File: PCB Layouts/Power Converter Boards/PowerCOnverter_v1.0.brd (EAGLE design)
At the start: 100 x 80 mm, 47 parts, among them Q1 PMBT3906, Q2 PMBT3906, Q3 PMBT3906, X1 48V, X2 12V, X3 24V, X4 15V

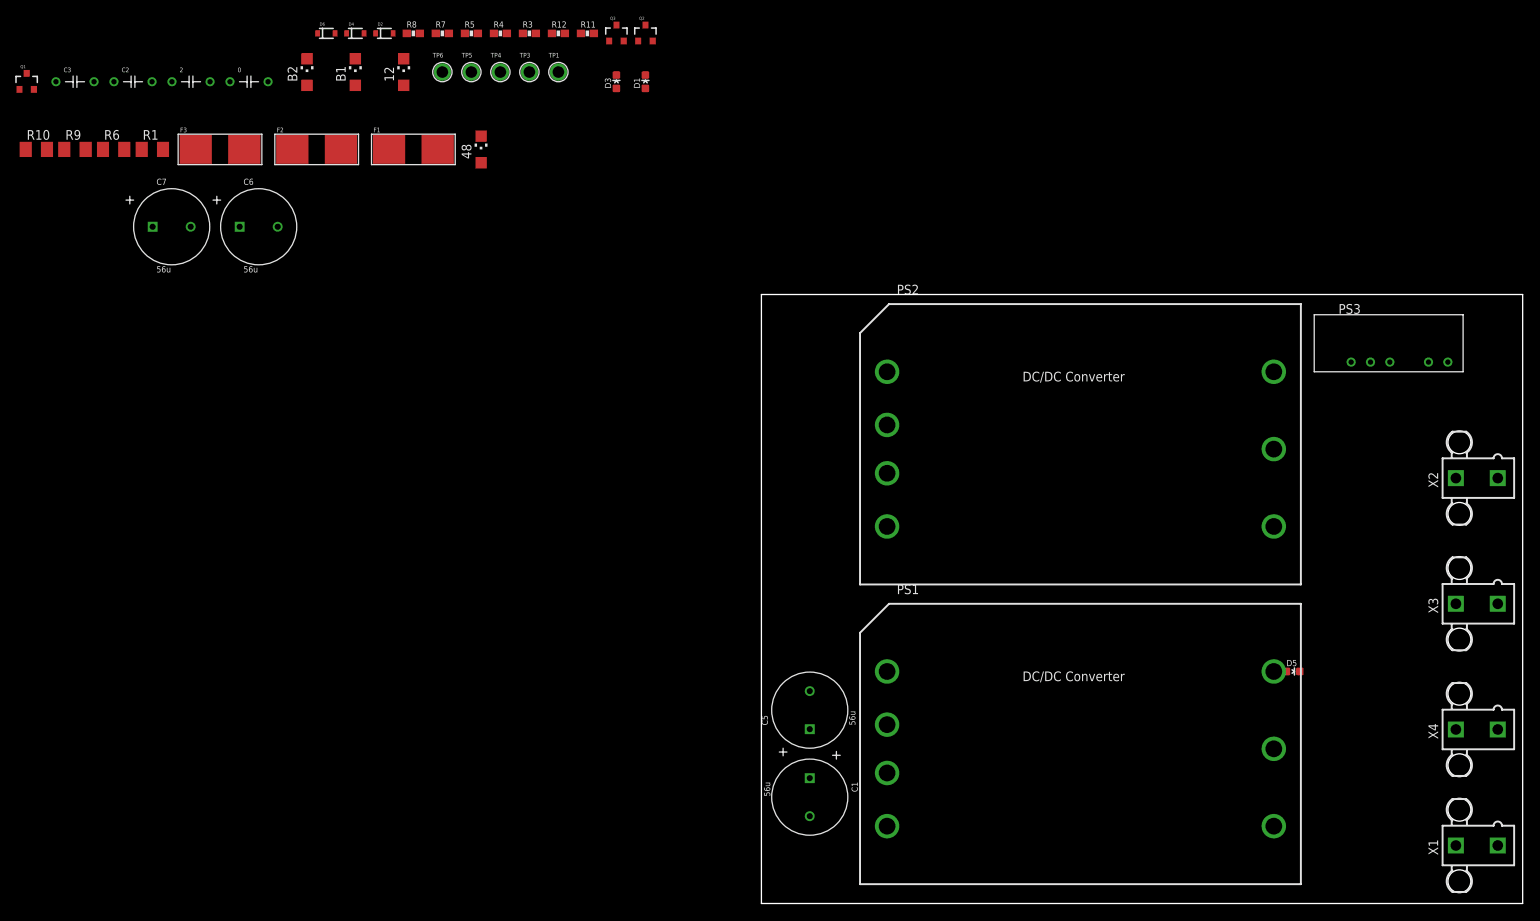
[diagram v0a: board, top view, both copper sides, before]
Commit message: MRAC adaptive control
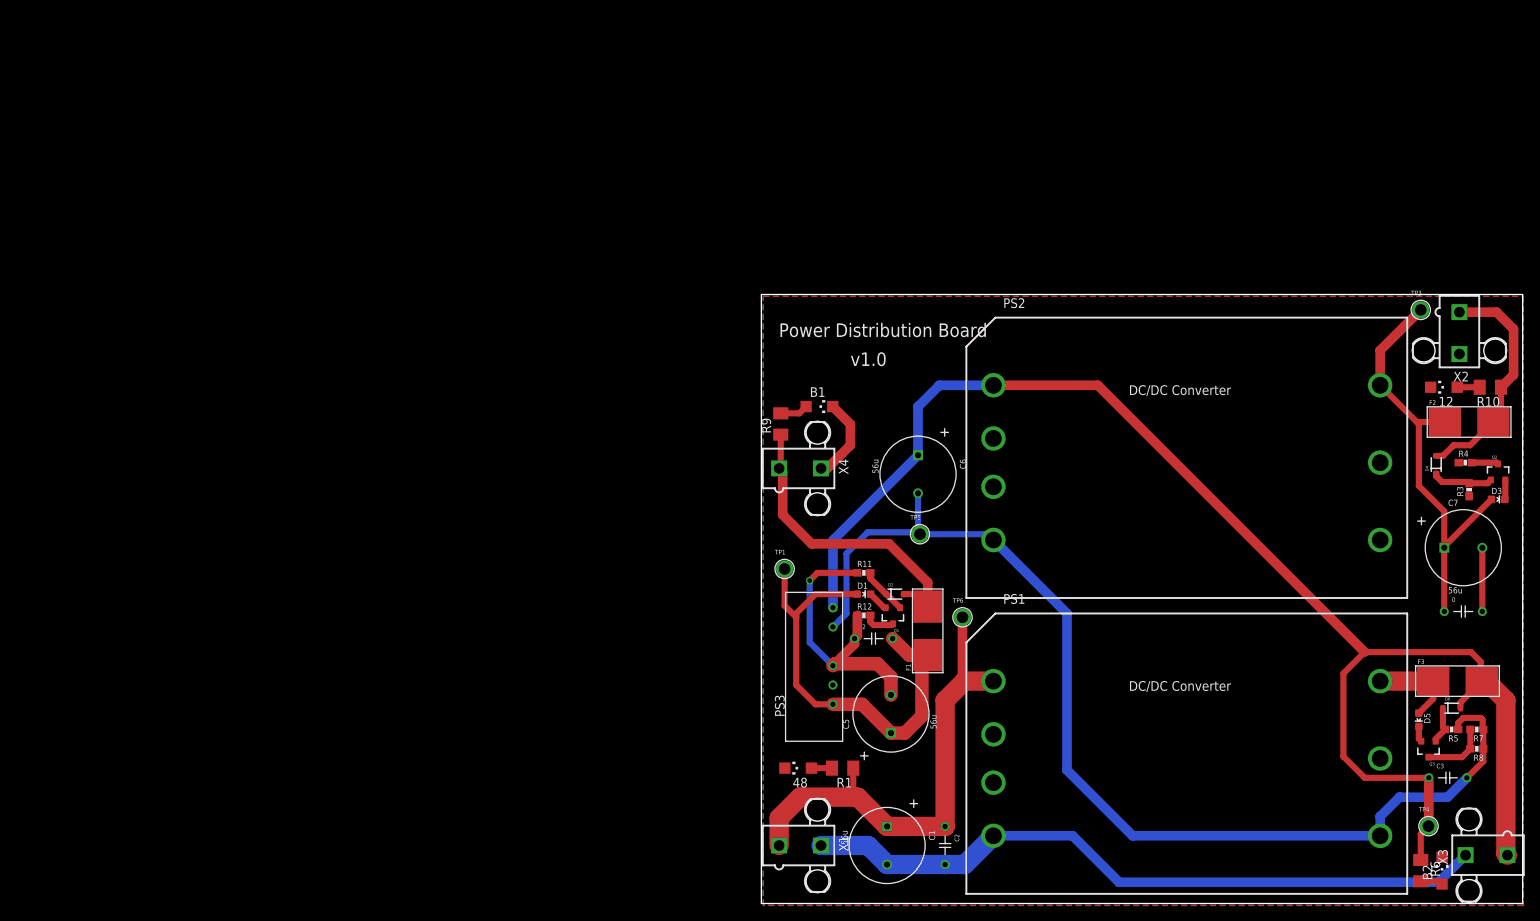
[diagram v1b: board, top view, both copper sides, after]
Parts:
- moved C3 202.2 mm to (90.2, 16.5)
- moved R6 196.1 mm to (86.6, 4.32), turned to 270 degrees
- moved R10 193.5 mm to (95.8, 67.8), turned to 180 degrees
- moved B2 182.3 mm to (89.4, 4.32)
- moved F3 176.9 mm to (91.4, 29.2)
- moved C7 174.8 mm to (92.2, 46.7)
- moved 0 174.0 mm to (92.2, 38.4)
- moved D6 172.4 mm to (90.7, 25.7)
- moved R8 168.4 mm to (94.0, 20.3), turned to 180 degrees
- moved R7 163.8 mm to (94.0, 22.9), turned to 180 degrees
- moved R5 157.9 mm to (90.7, 22.9), turned to 180 degrees
- moved TP4 157.1 mm to (87.6, 10.2)
- moved F2 155.6 mm to (93.0, 63.2)
- moved D4 152.9 mm to (88.6, 57.7), turned to 90 degrees
- moved C2 146.4 mm to (24.1, 7.62), turned to 270 degrees
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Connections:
- removed net 15V: X4.1
- removed net 24V: PS3.+VIN
- net +15V: now also X4.1
- net +24V: now also PS3.+VIN
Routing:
- net +24V: track 0.00 -> 191.6 mm
- net GND: track 0.00 -> 148.3 mm, vias 0 -> 1
- net -24V: track 0.00 -> 144.7 mm
- net 48V: track 0.00 -> 64.6 mm
- net +15V_OUT: track 0.00 -> 59.3 mm
- net N$8: track 0.00 -> 57.9 mm
- net +15V: track 0.00 -> 40.6 mm
- net +12V: track 0.00 -> 30.7 mm
- net N$3: track 0.00 -> 12.6 mm
- net N$6: track 0.00 -> 8.50 mm
- net N$11: track 0.00 -> 8.12 mm
- net N$20: track 0.00 -> 6.24 mm
- net N$12: track 0.00 -> 4.98 mm
- net N$19: track 0.00 -> 4.05 mm
- net N$13: track 0.00 -> 3.70 mm
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- added copper zone on layer 1, net GND
- added copper zone on layer 16, net GND
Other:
- board text added: "Power Distribution Board"
- board text added: "v1.0"
